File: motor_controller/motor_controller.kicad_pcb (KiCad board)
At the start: 4 copper layers, 30 x 62 mm, 139 parts, among them J1 etm, J2 Conn_01x06_MountingPin, J3 Conn_01x06_MountingPin, J4 Conn_01x03, U3 STM32G474VEHx

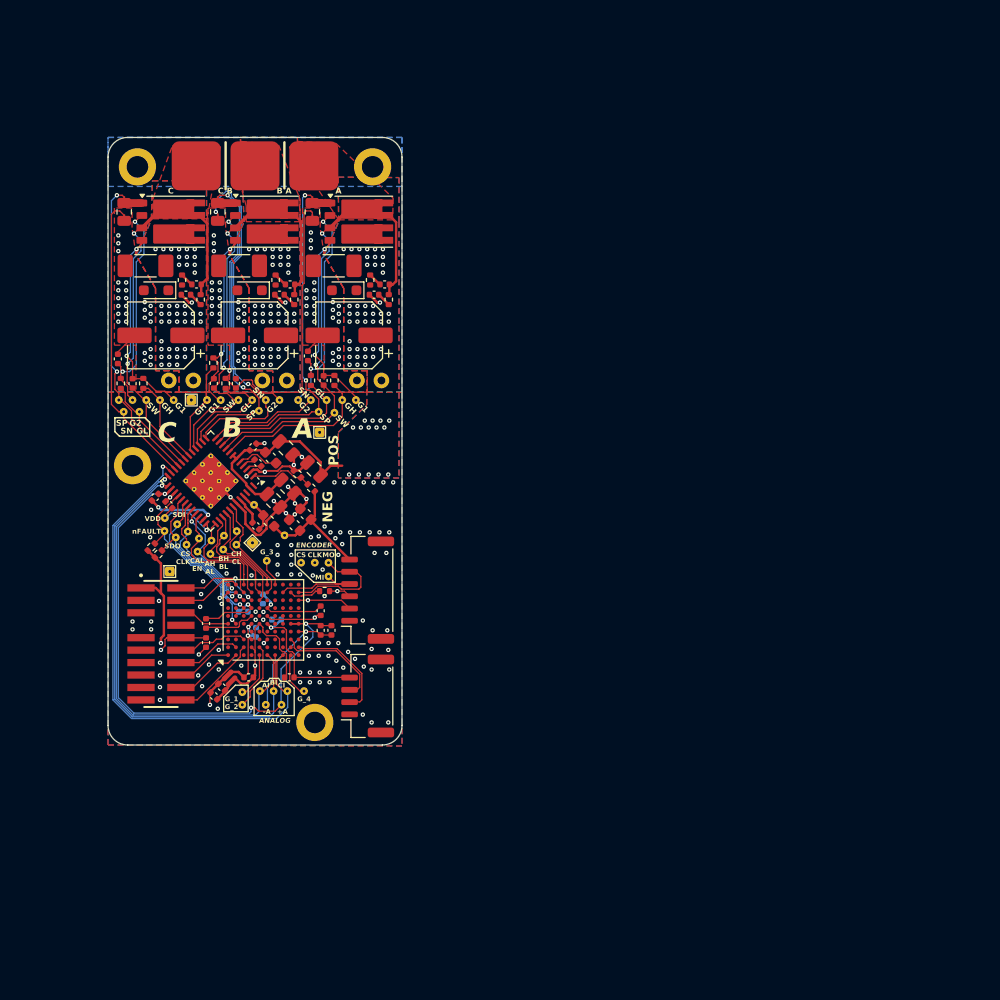
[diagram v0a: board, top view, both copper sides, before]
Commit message: still gotta put temp sensors on lol
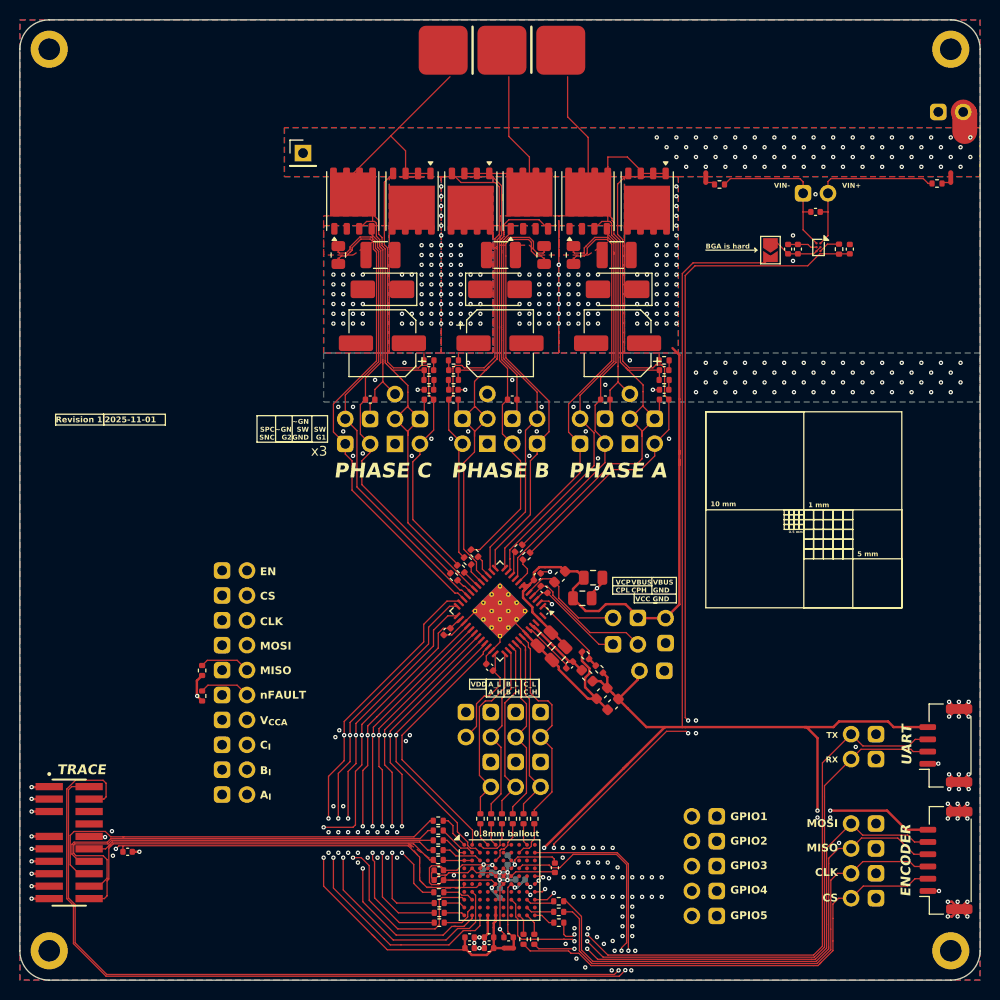
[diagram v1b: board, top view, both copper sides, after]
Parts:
- removed C21: ?, project:C_Disc_D3.0mm_W1.6mm_P2.50mm_no_silk
- removed TP24, TP25, TP26, TP27, TP28, TP29, TP30, TP31, TP32, TP33, TP34, TP45: test point, project:test point d1.5
- removed TP41, TP42, TP43, TP44: test point, project:ground test point d1.5
- added C47: 1u 6v3, Capacitor_SMD:C_0402_1005Metric, F.Cu at (98.4, 43.4)
- added C48: 1u 6v3, Capacitor_SMD:C_0402_1005Metric, F.Cu at (99.4, 43.4)
- added J5: Conn_01x03, project:tp_3x, F.Cu at (82.2, 63.2)
- added J6: Conn_01x03, project:tp_3x, F.Cu at (67.7, 63.2)
- added J7: Conn_01x03, project:tp_3x, F.Cu at (58.3, 63.3)
- added JP1: Jumper_2_Bridged, Jumper:SolderJumper-2_P1.3mm_Open_TrianglePad1.0x1.5mm, F.Cu at (96.6, 43.5)
- added NT3: NetTie_2, NetTie:NetTie-2_SMD_Pad0.5mm, F.Cu at (115.0, 36.1)
- added Q4: ~, Package_SON:Infineon_PG-TDSON-8_6.15x5.15mm, F.Cu at (84.0, 38.5)
- added Q5: ~, Package_SON:Infineon_PG-TDSON-8_6.15x5.15mm, F.Cu at (66.0, 38.5)
- added Q6: ~, Package_SON:Infineon_PG-TDSON-8_6.15x5.15mm, F.Cu at (60.0, 38.5)
- added R22: S10, Resistor_SMD:R_0402_1005Metric, F.Cu at (69.2, 101.5)
- added R23: S10, Resistor_SMD:R_0402_1005Metric, F.Cu at (67.0, 101.5)
- added R24: S10, Resistor_SMD:R_0402_1005Metric, F.Cu at (70.3, 101.5)
- added R25: S10, Resistor_SMD:R_0402_1005Metric, F.Cu at (68.1, 101.5)
- added R26: S10, Resistor_SMD:R_0402_1005Metric, F.Cu at (72.5, 101.5)
- added R27: S10, Resistor_SMD:R_0402_1005Metric, F.Cu at (71.4, 101.5)
- added R28: S10, Resistor_SMD:R_0402_1005Metric, F.Cu at (62.7, 105.7)
- added R29: S10, Resistor_SMD:R_0402_1005Metric, F.Cu at (62.7, 103.7)
- added R30: S10, Resistor_SMD:R_0402_1005Metric, F.Cu at (62.7, 101.7)
- added R31: S10, Resistor_SMD:R_0402_1005Metric, F.Cu at (62.7, 102.7)
- added R32: S10, Resistor_SMD:R_0402_1005Metric, F.Cu at (62.7, 104.7)
- added R33: S10, Resistor_SMD:R_0402_1005Metric, F.Cu at (71.4, 113.8)
- added R34: S10, Resistor_SMD:R_0402_1005Metric, F.Cu at (75.0, 111.0)
- added R35: S10, Resistor_SMD:R_0402_1005Metric, F.Cu at (75.0, 110.0)
- added R36: S10, Resistor_SMD:R_0402_1005Metric, F.Cu at (72.5, 113.8)
- added R37: S10, Resistor_SMD:R_0402_1005Metric, F.Cu at (62.8, 109.0)
- added R38: S10, Resistor_SMD:R_0402_1005Metric, F.Cu at (62.8, 110.1)
- added R39: S10, Resistor_SMD:R_0402_1005Metric, F.Cu at (62.8, 112.1)
- added R40: S10, Resistor_SMD:R_0402_1005Metric, F.Cu at (62.8, 111.1)
- added R41: S10, Resistor_SMD:R_0402_1005Metric, F.Cu at (75.0, 112.1)
- added R42: 100, Resistor_SMD:R_0402_1005Metric, F.Cu at (91.4, 36.8)
- added R43: S10, Resistor_SMD:R_0402_1005Metric, F.Cu at (103.6, 43.4)
- added TP55: test point, project:test point d1.5, F.Cu at (83.1, 83.7)
- added TP56: test point, project:test point d1.5, F.Cu at (80.5, 81.0)
- added TP57: test point, project:test point d1.5, F.Cu at (104.8, 95.4)
- added TP58: test point, project:test point d1.5, F.Cu at (85.9, 81.1)
- added TP59: test point, project:test point d1.5, F.Cu at (104.8, 92.9)
- added TP60: test point, project:test point d1.5, F.Cu at (88.6, 111.4)
- added U2: INA186A3IYFDR, project:TSBGA_0.4mm_flipped, F.Cu at (101.5, 43.2)
- C14, C2, C8: value ? -> 10u 50V; footprint Capacitor_SMD:C_1808_4520Metric -> Capacitor_SMD:C_1210_3225Metric
- C19: value ? -> 22nF; footprint project:C_Disc_D3.0mm_W1.6mm_P2.50mm_no_silk -> Capacitor_SMD:C_0402_1005Metric
- C20: footprint project:C_Disc_D3.0mm_W1.6mm_P2.50mm_no_silk -> Capacitor_SMD:C_0402_1005Metric
- D1, D2, D3: value 36 V -> 40 V; footprint Diode_SMD:D_SOD-323_HandSoldering -> Diode_SMD:D_SMA
- Q1, Q2, Q3: footprint project:BUK7V4R2-40HX -> Package_SON:Infineon_PG-TDSON-8_6.15x5.15mm
- R20: value 22 -> 100
- TP23: value test point -> TestPoint; footprint project:test point d1.5 -> Connector_PinHeader_2.54mm:PinHeader_1x01_P2.54mm_Vertical
- moved H2 99.4 mm to (115.0, 115.0)
- moved H1 83.9 mm to (115.0, 23.0)
- moved TP16 82.7 mm to (116.3, 29.4), turned to 180 degrees
- moved R20 75.1 mm to (113.6, 36.7), turned to 180 degrees
- moved TP14 73.2 mm to (102.5, 37.7), turned to 180 degrees
- moved NT2 70.6 mm to (90.0, 36.1), turned to 90 degrees
- moved TP50 65.7 mm to (104.8, 109.6)
- moved J2 65.1 mm to (114.5, 105.8)
- moved TP49 63.2 mm to (104.8, 107.1)
- moved TP48 60.1 mm to (104.8, 104.6)
- moved TP47 59.6 mm to (104.8, 102.0)
- moved J3 59.2 mm to (114.5, 94.0)
- moved C20 59.0 mm to (104.7, 43.4), turned to 90 degrees
- moved TP54 54.9 mm to (88.6, 108.9), turned to 0 degrees
- moved TP53 48.7 mm to (88.6, 106.4), turned to 0 degrees
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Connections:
- net Net-(U1C-CPH) renamed /CPH
- net Net-(U1C-CPL) renamed /CPL
- net Net-(U1C-VCP) renamed /VCP
- C10 pad 2: GND -> /Phase B/GND_ISH
- C16 pad 2: GND -> /Phase C/GND_ISH
- C19 pad 1: VBUS -> /VIN+
- C19 pad 2: GND -> /VIN-
- C20 pad 1: VBUS -> /CURR_SENSE_OUTPUT
- C27 pad 2: VSSA -> GND
- C38 pad 2: VSSA -> GND
- C39 pad 2: VSSA -> GND
- C4 pad 2: GND -> /Phase A/GND_ISH
- C45 pad 2: VSSA -> GND
- C46 pad 2: VSSA -> GND
- J1 pad 11: unconnected-(J1-GND-Pad11) -> GND
- J1 pad 6: /SWO -> unconnected-(J1-SWO/TDO-Pad6)
- J3 pad 2: /UART_TX -> /UART_RX
- J3 pad 3: /UART_RX -> /UART_TX
- NT2 pad 1: VSSA -> Net-(NT2-Pad1)
- NT2 pad 2: GND -> VBUS
- Q1 pad 1: Net-(Q1-S2) -> /Phase A/GND_ISH
- Q1 pad 2: /Phase A/G2 -> /Phase A/GND_ISH
- Q1 pad 3: /A_SW -> /Phase A/GND_ISH
- Q1 pad 4: /Phase A/G1 -> /Phase A/G2
- Q1 pad 5: VBUS -> /A_SW
- Q2 pad 1: Net-(Q2-S2) -> /Phase B/GND_ISH
- Q2 pad 2: /Phase B/G2 -> /Phase B/GND_ISH
- Q2 pad 3: /B_SW -> /Phase B/GND_ISH
- Q2 pad 4: /Phase B/G1 -> /Phase B/G2
- Q2 pad 5: VBUS -> /B_SW
- Q3 pad 1: Net-(Q3-S2) -> /Phase C/GND_ISH
- Q3 pad 2: /Phase C/G2 -> /Phase C/GND_ISH
- Q3 pad 3: /C_SW -> /Phase C/GND_ISH
- Q3 pad 4: /Phase C/G1 -> /Phase C/G2
- Q3 pad 5: VBUS -> /C_SW
- R14 pad 1: /SDO -> /DRV_MISO
- R16 pad 4: Net-(Q1-S2) -> /Phase A/GND_ISH
- R17 pad 4: Net-(Q2-S2) -> /Phase B/GND_ISH
- R18 pad 4: Net-(Q3-S2) -> /Phase C/GND_ISH
- R20 pad 1: Net-(U3-PB13) -> Net-(NT3-Pad1)
- R20 pad 2: /ENC_CLK -> /VIN+
- TP1 pad 1: /A_L -> /A_H
- TP10 pad 1: /SDO -> /DRV_MISO
- TP11 pad 1: /SDI -> /DRV_MOSI
- TP12 pad 1: /SCLK -> /DRV_CLK
- TP13 pad 1: /SPI_NSS -> /DRV_CS
- TP14 pad 1: /CAL -> /VIN+
- TP16 pad 1: Net-(U1B-SW) -> VBUS
- TP2 pad 1: /B_L -> /B_H
- TP20 pad 1: Net-(U1D-SNA) -> Net-(U1D-SPA)
- TP21 pad 1: Net-(U1E-SNB) -> Net-(U1E-SPB)
- TP22 pad 1: Net-(U1F-SNC) -> Net-(U1F-SPC)
- TP23 pad 1: Net-(U1D-SPA) -> VBUS
- TP3 pad 1: /C_L -> /C_H
- TP4 pad 1: /A_H -> /A_L
- TP5 pad 1: /B_H -> /B_L
- TP51 pad 1: /GPIO_4 -> /GPIO1
- TP52 pad 1: /GPIO_1 -> /GPIO2
- TP53 pad 1: /GPIO_2 -> /GPIO3
- TP54 pad 1: /GPIO_3 -> /GPIO4
- TP6 pad 1: /C_H -> /C_L
- U1 pad 29: /SDO -> /DRV_MISO
- U1 pad 30: /SDI -> /DRV_MOSI
- U1 pad 31: /SCLK -> /DRV_CLK
- U1 pad 32: /SPI_NSS -> /DRV_CS
- U1 pad 35: VSSA -> GND
- U3 pad A1: /TRACE1 -> /T1
- U3 pad A10: /EN -> unconnected-(U3-PC12-PadA10)
- U3 pad A2: unconnected-(U3-PB9-PadA2) -> /CAL
- U3 pad A3: unconnected-(U3-PB8-PadA3) -> Net-(U3-PB8)
- U3 pad A4: unconnected-(U3-PB6-PadA4) -> Net-(U3-PB6)
- U3 pad A5: /SWO -> Net-(U3-PB3)
- U3 pad A9: /nFAULT -> Net-(U3-PD1)
- U3 pad B1: /TRACE2 -> /T2
- U3 pad B2: /TRACE0 -> /T0
- U3 pad B3: unconnected-(U3-PE1-PadB3) -> /EN
- U3 pad B5: /SDI -> unconnected-(U3-PB5-PadB5)
- U3 pad B8: unconnected-(U3-PD0-PadB8) -> Net-(U3-PD0)
- U3 pad B9: /SPI_NSS -> unconnected-(U3-PA15-PadB9)
- U3 pad C1: unconnected-(U3-PC14-PadC1) -> /T3
- U3 pad C10: /A_H -> unconnected-(U3-PA11-PadC10)
- U3 pad C2: /TRACE3 -> /T3
- U3 pad C3: /TRACECLK -> Net-(U3-PE2)
- U3 pad C5: unconnected-(U3-PB4-PadC5) -> Net-(U3-PB4)
- U3 pad C7: /SDO -> unconnected-(U3-PC11-PadC7)
- U3 pad C8: /SCLK -> unconnected-(U3-PC10-PadC8)
- U3 pad C9: /CAL -> unconnected-(U3-PA12-PadC9)
- U3 pad D9: /A_L -> unconnected-(U3-PA10-PadD9)
- U3 pad E1: /GPIO_1 -> unconnected-(U3-PF0-PadE1)
- U3 pad E10: unconnected-(U3-PA8-PadE10) -> /CURR_SENSE_OUTPUT
- U3 pad E2: /GPIO_2 -> unconnected-(U3-PF1-PadE2)
- U3 pad E8: /B_L -> unconnected-(U3-PC8-PadE8)
- U3 pad E9: /B_H -> unconnected-(U3-PC9-PadE9)
- U3 pad F1: /A_I -> unconnected-(U3-PC2-PadF1)
- U3 pad F10: /C_H -> /GPIO1
- U3 pad F9: /C_L -> /GPIO2
- U3 pad G1: /B_I -> unconnected-(U3-PC3-PadG1)
- U3 pad G10: /GPIO_3 -> /GPIO3
- U3 pad G2: unconnected-(U3-PA1-PadG2) -> /B_I
- U3 pad G9: unconnected-(U3-PD13-PadG9) -> /GPIO4
- U3 pad H1: /C_I -> /A_I
- U3 pad H10: unconnected-(U3-PD11-PadH10) -> /GPIO5
- U3 pad H2: unconnected-(U3-PA4-PadH2) -> Net-(U3-PA4)
- U3 pad H7: unconnected-(U3-PE15-PadH7) -> /UART_RX
- U3 pad H9: /ENC_MISO -> Net-(U3-PB14)
- U3 pad J1: /GPIO_4 -> Net-(U3-PA5)
- U3 pad J2: unconnected-(U3-PA6-PadJ2) -> Net-(U3-PA6)
- U3 pad J3: /UART_RX -> unconnected-(U3-PC5-PadJ3)
- U3 pad K1: unconnected-(U3-PA7-PadK1) -> Net-(U3-PA7)
- U3 pad K10: unconnected-(U3-PD8-PadK10) -> Net-(U3-PD8)
- U3 pad K2: /UART_TX -> /nFAULT
- U3 pad K3: unconnected-(U3-PB1-PadK3) -> /C_I
- U3 pad K4: VSSA -> GND
- U3 pad K8: /ENC_CS -> Net-(U3-PB12)
- U3 pad K9: /ENC_MOSI -> Net-(U3-PB15)
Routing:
- net VCC: track 92.6 -> 289.6 mm, vias 6 -> 10
- net /SWCLK: track 6.56 -> 102.7 mm, vias 0 -> 2
- net /SWDIO: track 8.90 -> 98.5 mm
- net /CURR_SENSE_OUTPUT: track 0.00 -> 87.8 mm, vias 0 -> 4
- net GND: track 73.8 -> 146.7 mm, vias 186 -> 288
- net VSSA: track 62.3 -> 0.00 mm, vias 4 -> 0
- net /DRV_MISO: track 0.00 -> 59.6 mm, vias 0 -> 3
- net /DRV_CLK: track 0.00 -> 54.4 mm, vias 0 -> 3
- net /DRV_MOSI: track 0.00 -> 54.3 mm, vias 0 -> 3
- net /UART_RX: track 11.3 -> 65.3 mm, vias 0 -> 2
- net /DRV_CS: track 0.00 -> 52.6 mm, vias 0 -> 3
- net /UART_TX: track 11.6 -> 60.5 mm, vias 0 -> 2
- net /nFAULT: track 17.3 -> 65.6 mm, vias 1 -> 3
- net /ENC_CLK: track 6.13 -> 49.9 mm, vias 1 -> 0
- net /ENC_MISO: track 9.62 -> 53.0 mm
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- added copper zone on F.Cu, net /Phase A/GND_ISH
- added copper zone on F.Cu, net /Phase B/GND_ISH
- added copper zone on F.Cu, net /Phase C/GND_ISH
- added copper zone on In1.Cu, net VBUS
- added copper zone on In2.Cu, net VBUS
- added copper zone on F.Cu, net VCC
- removed copper zone on F.Cu, net /A_SW
- removed copper zone on F.Cu, net /B_SW
- removed copper zone on F.Cu, net /C_SW
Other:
- board size 30 x 62 mm -> 98 x 98 mm
- board text added: "0.5 mm"
- board text added: "0.8mm ballout"
- board text added: "1 mm"
- board text added: "10 mm"
- board text added: "2025-11-01"
- board text added: "5 mm"
- board text added: "A_L A_H"
- board text added: "A_{I}"
- board text added: "BGA is hard"
- board text added: "B_L B_H"
- board text added: "B_{I}"
- board text added: "CARSON 'VERTER"
- board text added: "C_L C_H"
- board text added: "C_{I}"
- board text added: "EN"
- board text added: "GPIO1"
- board text added: "GPIO2"
- board text added: "GPIO3"
- board text added: "GPIO4"
- board text added: "GPIO5"
- board text added: "MISO"
- board text added: "MOSI"
- board text added: "PHASE A"
- board text added: "PHASE B"
- board text added: "PHASE C"
- board text added: "RX"
- board text added: "Revision 1"
- board text added: "SPC SNC"
- board text added: "SW G1"
- board text added: "TRACE"
- board text added: "TX"
- board text added: "UART"
- board text added: "VBUS CPH"
- board text added: "VBUS GND"
- board text added: "VCC GND"
- board text added: "VCP CPL"
- board text added: "VIN+"
- board text added: "VIN-"
- board text added: "V_{CCA}"
- board text added: "x3"
- board text added: "~GN G2"
- board text added: "~GN SW GND"
- board text removed: "+A"
- board text removed: "-A"
- board text removed: "A"
- board text removed: "AH AL"
- board text removed: "AI"
- board text removed: "ANALOG"
- board text removed: "B"
- board text removed: "BH BL"
- board text removed: "BI"
- board text removed: "C"
- board text removed: "CAL EN"
- board text removed: "CH CL"
- board text removed: "CI"
- board text removed: "CS CLK"
- board text removed: "G1"
- board text removed: "G2"
- board text removed: "GH"
- board text removed: "GL"
- board text removed: "G_1"
- board text removed: "G_2"
- board text removed: "G_3"
- board text removed: "G_4"
- board text removed: "MI"
- board text removed: "MO"
- board text removed: "NEG"
- board text removed: "POS"
- board text removed: "SDI"
- board text removed: "SDO"
- board text removed: "SN"
- board text removed: "SP"
- board text removed: "SW"
